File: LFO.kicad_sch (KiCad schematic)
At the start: 9 parts, among them U2 RC4558

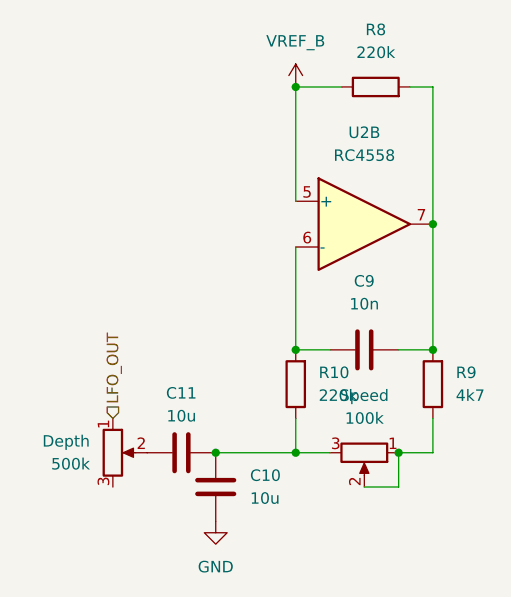
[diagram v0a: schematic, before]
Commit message: finalise schems for now
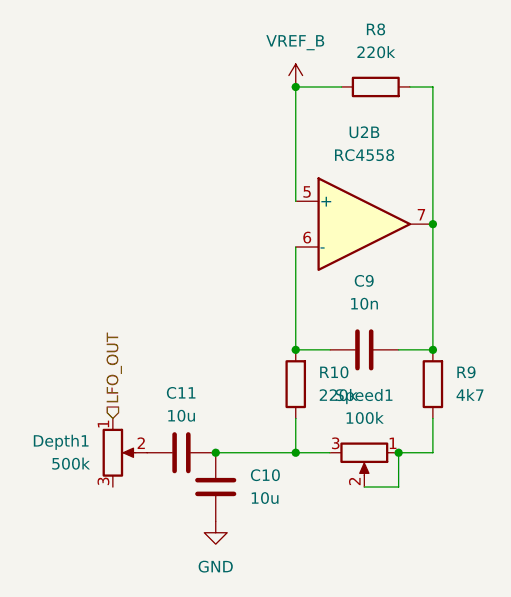
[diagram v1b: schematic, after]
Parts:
- C10, C11, C9: footprint (none) -> Capacitor_SMD:C_0805_2012Metric
- Depth1: renamed from Depth; footprint (none) -> Connector_PinHeader_2.54mm:PinHeader_1x02_P2.54mm_Vertical
- R10, R8, R9: footprint (none) -> Resistor_SMD:R_0805_2012Metric
- Speed1: renamed from Speed; footprint (none) -> Potentiometer_THT:Potentiometer_Alpha_RD902F-40-00D_Dual_Vertical
- U2: footprint (none) -> Package_SO:SOIC-8W_5.3x5.3mm_P1.27mm
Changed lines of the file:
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@@
 			)
 		)
-		(property "Footprint" ""
+		(property "Footprint" "Resistor_SMD:R_0805_2012Metric"
 			(at 88.138 129.54 90)
 			(effects
@@
 			)
 		)
-		(property "Footprint" ""
+		(property "Footprint" "Resistor_SMD:R_0805_2012Metric"
 			(at 95.25 98.298 90)
 			(effects
@@
 		(dnp no)
 		(fields_autoplaced yes)
-		(property "Reference" "Speed"
+		(property "Reference" "Speed1"
 			(at 93.98 130.81 90)
 			(effects
@@
 			)
 		)
-		(property "Footprint" ""
+		(property "Footprint" "Potentiometer_THT:Potentiometer_Alpha_RD902F-40-00D_Dual_Vertical"
 			(at 93.98 137.16 0)
 			(effects
@@
 			(project "lofi-chorus"
 				(path "/588a825c-d767-4731-8ddd-93a0322145f3/ad47ec63-ab79-496c-acf3-001c089e7238"
-					(reference "Speed")
+					(reference "Speed1")
 					(unit 1)
 				)
@@
 			)
 		)
-		(property "Footprint" ""
+		(property "Footprint" "Capacitor_SMD:C_0805_2012Metric"
 			(at 97.79 124.7648 0)
 			(effects
@@
 			)
 		)
-		(property "Footprint" ""
+		(property "Footprint" "Capacitor_SMD:C_0805_2012Metric"
 			(at 76.5048 137.16 0)
 			(effects
@@
 			)
 		)
-		(property "Footprint" ""
+		(property "Footprint" "Capacitor_SMD:C_0805_2012Metric"
 			(at 69.85 138.1252 0)
 			(effects
@@
 			)
 		)
-		(property "Footprint" ""
+		(property "Footprint" "Resistor_SMD:R_0805_2012Metric"
 			(at 103.378 129.54 90)
 			(effects
@@
 			)
 		)
-		(property "Footprint" ""
+		(property "Footprint" "Package_SO:SOIC-8W_5.3x5.3mm_P1.27mm"
 			(at 93.98 111.76 0)
 			(effects
@@
 		(dnp no)
 		(fields_autoplaced yes)
-		(property "Reference" "Depth"
+		(property "Reference" "Depth1"
 			(at 63.5 135.8899 0)
 			(effects
@@
 			)
 		)
-		(property "Footprint" ""
+		(property "Footprint" "Connector_PinHeader_2.54mm:PinHeader_1x02_P2.54mm_Vertical"
 			(at 66.04 137.16 0)
 			(effects
@@
 			(project "lofi-chorus"
 				(path "/588a825c-d767-4731-8ddd-93a0322145f3/ad47ec63-ab79-496c-acf3-001c089e7238"
-					(reference "Depth")
-					(unit 1)
-				)
+					(reference "Depth1")
+					(unit 1)
+				)
